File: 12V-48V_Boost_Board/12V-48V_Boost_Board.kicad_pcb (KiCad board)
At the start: 2 copper layers, 31 parts, among them J1 12V Input, J2 Input Current Sensing, J3 Output Current Sensing, J4 48V Output, Q1 100V

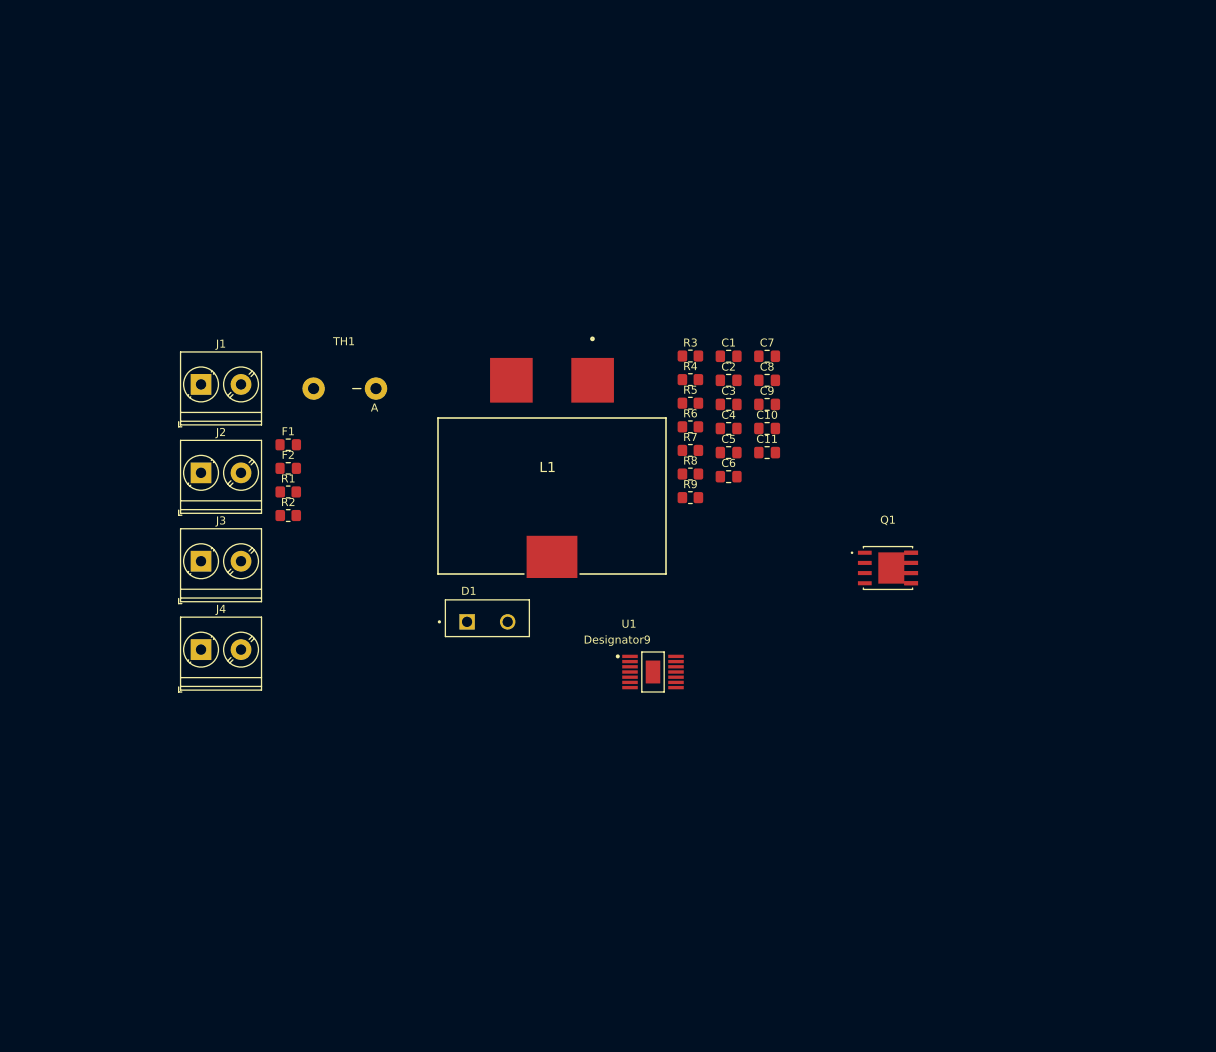
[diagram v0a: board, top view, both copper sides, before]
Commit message: First attempt in the pcb layout and routing
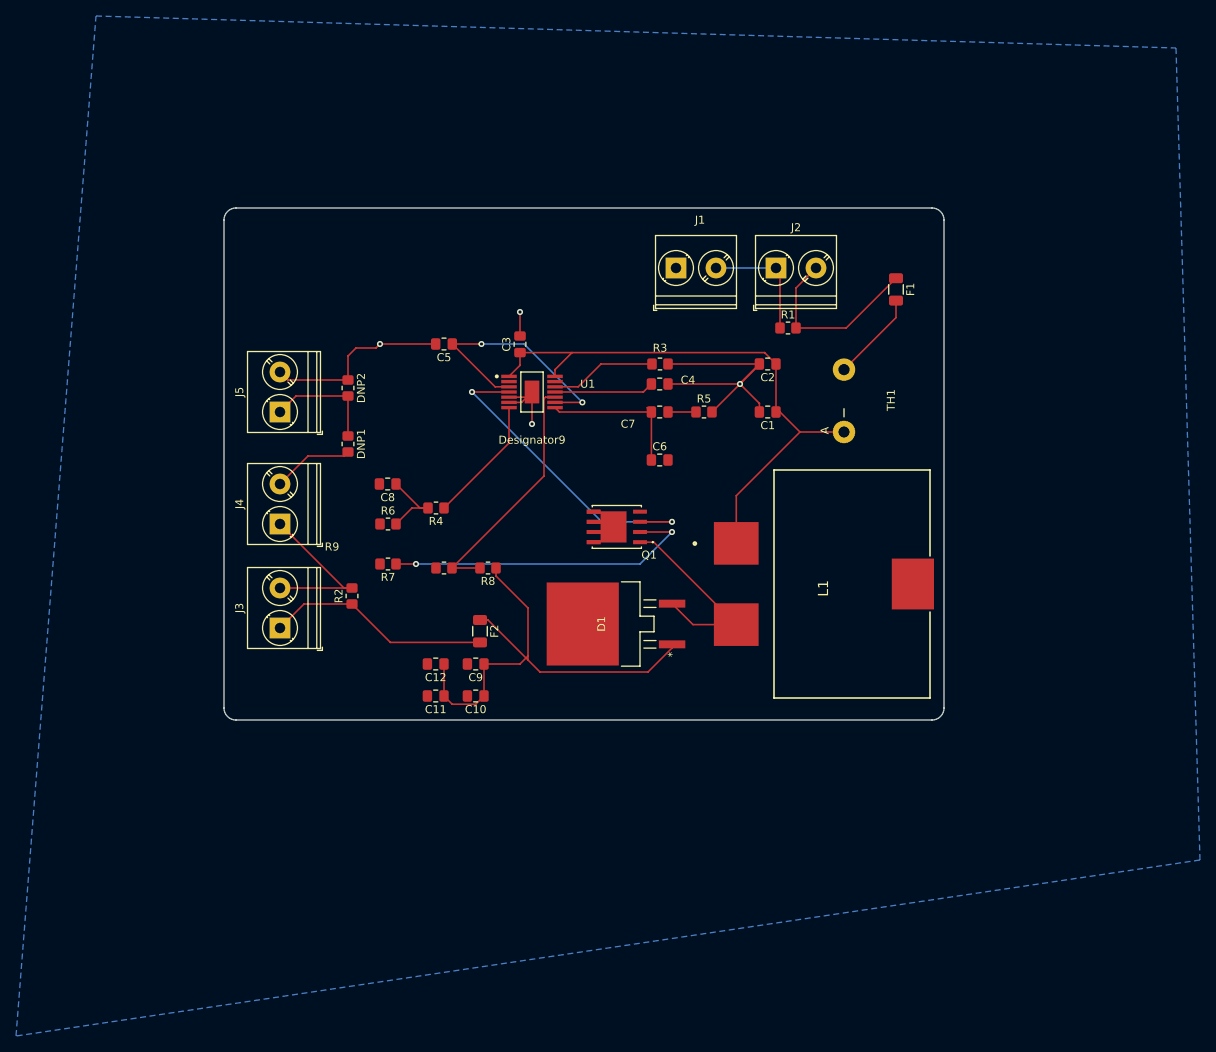
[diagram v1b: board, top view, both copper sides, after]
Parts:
- added C12: 1µF, Capacitor_SMD:C_0805_2012Metric_Pad1.18x1.45mm_HandSolder, F.Cu at (136.5, 128.0)
- added DNP1: 1mΩ, Resistor_SMD:R_0805_2012Metric_Pad1.20x1.40mm_HandSolder, F.Cu at (125.5, 100.5)
- added DNP2: ~, Resistor_SMD:R_0805_2012Metric_Pad1.20x1.40mm_HandSolder, F.Cu at (125.5, 93.5)
- added J5: Output Measuring, TerminalBlock_Phoenix:TerminalBlock_Phoenix_PT-1,5-2-5.0-H_1x02_P5.00mm_Horizontal, F.Cu at (117.0, 96.5)
- C11: value 1µF -> 10µF
- C2: value 100nF -> 4.7µF
- C3: value 63nF -> 100nF
- C4: value 1µF -> 63nF
- C5: value 120nF -> 1µF
- C6: value 100nF -> 120nF
- C7: value 1nF -> 100nF
- C8: value 10µF -> 1nF
- D1: value 800mV -> 455mV; footprint Library:TO-220-2 -> 12/48 boost:D2PAK_STM-M
- F1: footprint Fuse:Fuse_0805_2012Metric_Pad1.15x1.40mm_HandSolder -> Fuse:Fuse_1206_3216Metric
- F2: value 3A -> 2A; footprint Fuse:Fuse_0805_2012Metric_Pad1.15x1.40mm_HandSolder -> Fuse:Fuse_1206_3216Metric
- L1: footprint Library:WE-HCF_SMD_HIGH-CURRENT_INDUCTOR -> 12/48 boost:WE-HCF_SMD_HIGH-CURRENT_INDUCTOR
- Q1: value 100V -> FDWS86068-F085; footprint Library:Q1 Mosfet -> 12/48 boost:Q1 Mosfet
- TH1: footprint Library:Inrush Current Limiter -> 12/48 boost:Inrush Current Limiter
- U1: footprint Library:LM5156H -> 12/48 boost:LM5156H
- moved F1 78.4 mm to (194.0, 81.2), turned to -90 degrees
- moved J2 76.3 mm to (179.0, 78.5)
- moved TH1 66.3 mm to (187.5, 91.2), turned to -90 degrees
- moved R1 65.7 mm to (180.5, 86.0)
- moved J1 61.1 mm to (166.5, 78.5)
- moved C11 51.4 mm to (136.5, 132.0), turned to 180 degrees
- moved C10 49.4 mm to (141.5, 132.0), turned to 180 degrees
- moved C8 49.2 mm to (130.5, 105.5), turned to 180 degrees
- moved C9 48.8 mm to (141.5, 128.0), turned to 180 degrees
- moved R7 40.4 mm to (130.5, 115.5), turned to 180 degrees
- moved R6 39.7 mm to (130.5, 110.5)
- moved L1 39.1 mm to (188.5, 118.0), turned to 90 degrees
- moved U1 38.1 mm to (148.5, 94.0)
- moved C5 38.1 mm to (137.5, 88.0), turned to 180 degrees
- moved R4 35.6 mm to (136.5, 108.5), turned to 180 degrees
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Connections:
- C10 pad 1: Net-(C10-Pad1) -> /Boost_Board_Chip/48V_OUTPUT
- C3 pad 1: Net-(U1-SS) -> /Boost_Board_Chip/12V_INPUT
- C4 pad 1: /Boost_Board_Chip/DITHOFF -> Net-(U1-SS)
- C5 pad 1: Net-(U1-COMP) -> /Boost_Board_Chip/DITHOFF
- C6 pad 2: Net-(C6-Pad2) -> GND
- C7 pad 1: Net-(C7-Pad1) -> Net-(U1-COMP)
- C7 pad 2: GND -> Net-(C7-Pad2)
- C8 pad 1: /Boost_Board_Chip/48V_OUTPUT -> Net-(C8-Pad1)
- C8 pad 2: Net-(C8-Pad2) -> GND
- C9 pad 1: Net-(C8-Pad2) -> /Boost_Board_Chip/48V_OUTPUT
- C9 pad 2: Net-(C10-Pad1) -> GND
- J4 pad 2: GND -> Net-(J4-Pin_2)
- Q1 pad 2: Net-(Q1-G) -> Net-(Q1-S)
- Q1 pad 3: Net-(Q1-S) -> Net-(Q1-G)
- R4 pad 2: Net-(C7-Pad1) -> Net-(C8-Pad1)
- R5 pad 1: Net-(C6-Pad2) -> Net-(C7-Pad2)
- R6 pad 2: Net-(C7-Pad1) -> Net-(C8-Pad1)
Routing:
- net GND: track 0.00 -> 74.0 mm, vias 0 -> 4
- net /Boost_Board_Chip/12V_INPUT: track 0.00 -> 72.7 mm
- net /Boost_Board_Chip/48V_OUTPUT: track 0.00 -> 61.3 mm
- net Net-(Q1-G): track 0.00 -> 40.3 mm, vias 0 -> 2
- net Net-(Q1-S): track 0.00 -> 40.2 mm, vias 0 -> 2
- net /Boost_Board_Chip/DITHOFF: track 0.00 -> 32.0 mm, vias 0 -> 2
- net Net-(U1-FB): track 0.00 -> 30.9 mm
- net Net-(J3-Pin_1): track 0.00 -> 28.2 mm
- net Net-(D1-A): track 0.00 -> 25.4 mm
- net Net-(J2-Pin_2): track 0.00 -> 23.6 mm
- net Net-(J3-Pin_2): track 0.00 -> 21.3 mm
- net Net-(U1-COMP): track 0.00 -> 19.1 mm
- net Net-(U1-CS): track 0.00 -> 15.9 mm
- net Net-(J1-Pin_2): track 0.00 -> 15.2 mm
- net Net-(J5-Pin_1): track 0.00 -> 14.3 mm
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- added copper zone on B.Cu, net GND
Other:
- board outline added: 90 x 64 mm
